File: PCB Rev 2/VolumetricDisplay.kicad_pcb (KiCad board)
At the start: 4 copper layers, 48.5 x 56 mm, 149 parts, among them J1 USB_C_Receptacle_USB2.0_16P, J2 Conn_ARM_SWD_TagConnect_TC2030, Q1 DMN32D2LDF, Q2 DMN32D2LDF, Q3 DMN32D2LDF, Q4 DMN32D2LDF, SW4 TS-1088-AR02016, SW5 TS-1088-AR02016, U2 NCP718xSN330, U3 RP2354B, U4 DRV8311S, U5 DRV5055A1xDBZxQ1, Y1 Abracon ABM8-272-T3

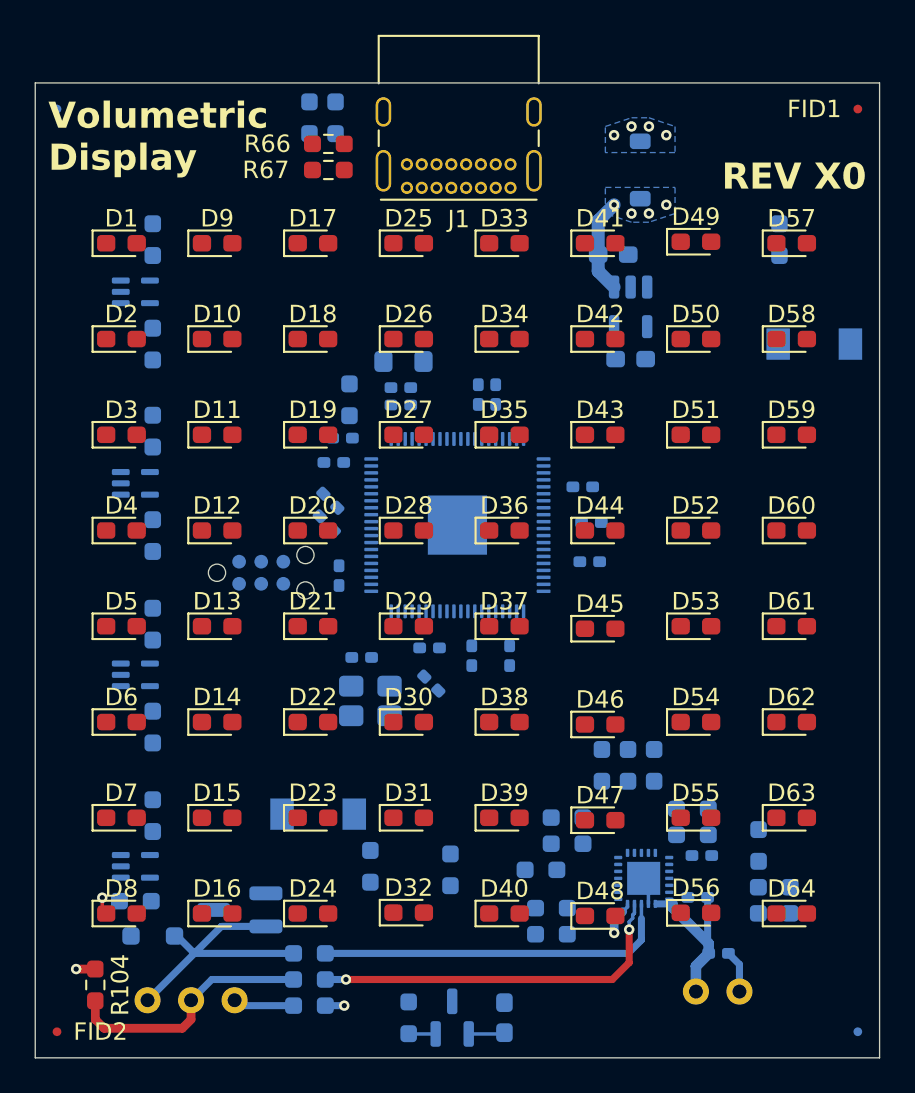
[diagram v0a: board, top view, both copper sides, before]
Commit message: Started traces
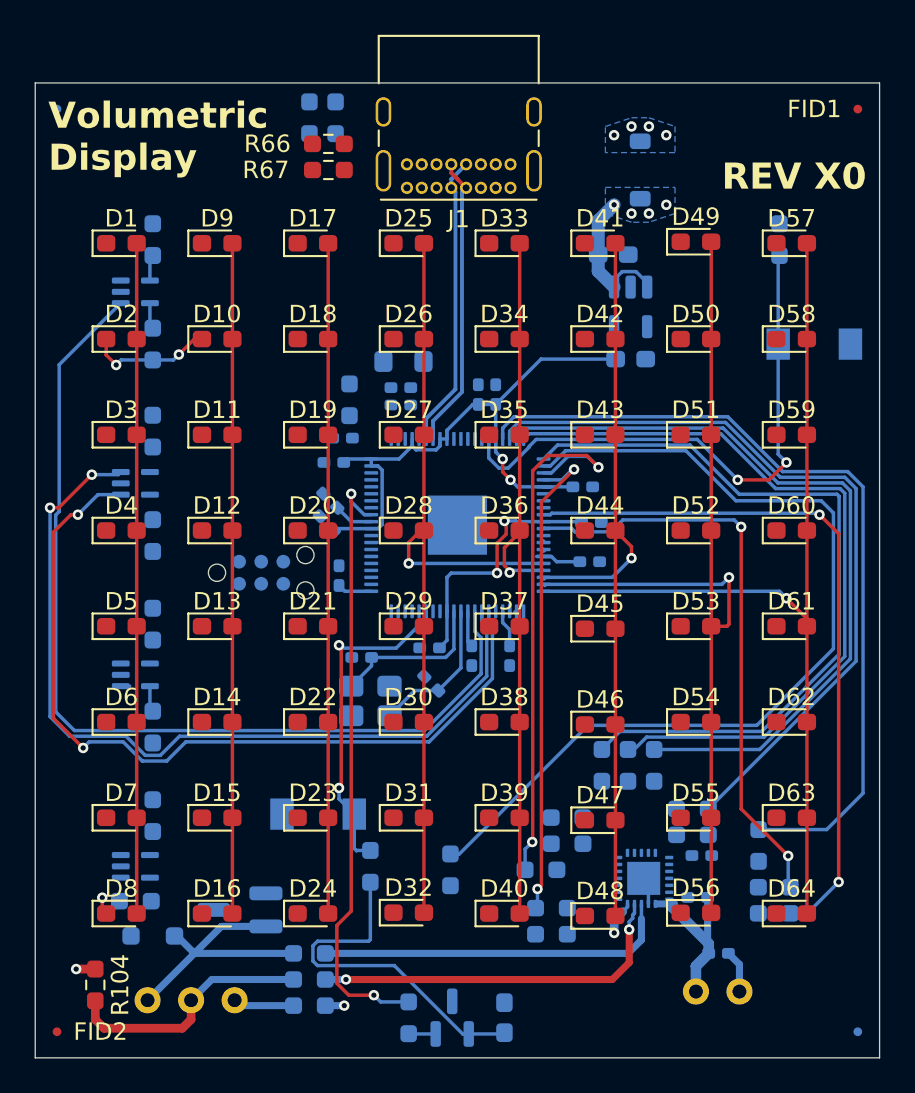
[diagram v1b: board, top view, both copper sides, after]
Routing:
- net 3V3: track 2.08 -> 64.9 mm, vias 0 -> 2
- net LED9: track 0.00 -> 55.0 mm
- net LED7: track 0.00 -> 54.7 mm, vias 0 -> 1
- net LED6: track 0.00 -> 53.2 mm, vias 0 -> 1
- net Net-(U3-GPIO5): track 0.00 -> 53.2 mm
- net LED10: track 0.00 -> 48.6 mm, vias 0 -> 2
- net LED3: track 0.00 -> 48.6 mm, vias 0 -> 1
- net LED11: track 0.00 -> 47.9 mm, vias 0 -> 2
- net Net-(U3-GPIO0): track 0.00 -> 47.7 mm
- net LED5: track 0.00 -> 46.2 mm, vias 0 -> 1
- net Net-(U3-GPIO2): track 0.00 -> 44.2 mm
- net Net-(U3-GPIO1): track 0.00 -> 44.0 mm
- net Net-(U3-GPIO3): track 0.00 -> 44.0 mm
- net Net-(U3-GPIO4): track 0.00 -> 43.5 mm
- net LED4: track 0.00 -> 43.4 mm, vias 0 -> 1
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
